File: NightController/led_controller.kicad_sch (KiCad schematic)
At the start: 22 parts, among them U301 LP5036, U302 EAST1410RGBW02, U303 EAST1410RGBW02, U304 EAST1410RGBW02, U305 EAST1410RGBW02, U306 EAST1410RGBW02, U307 EAST1410RGBW02, U308 EAST1410RGBW02, U309 EAST1410RGBW02, U310 EAST1410RGBW02

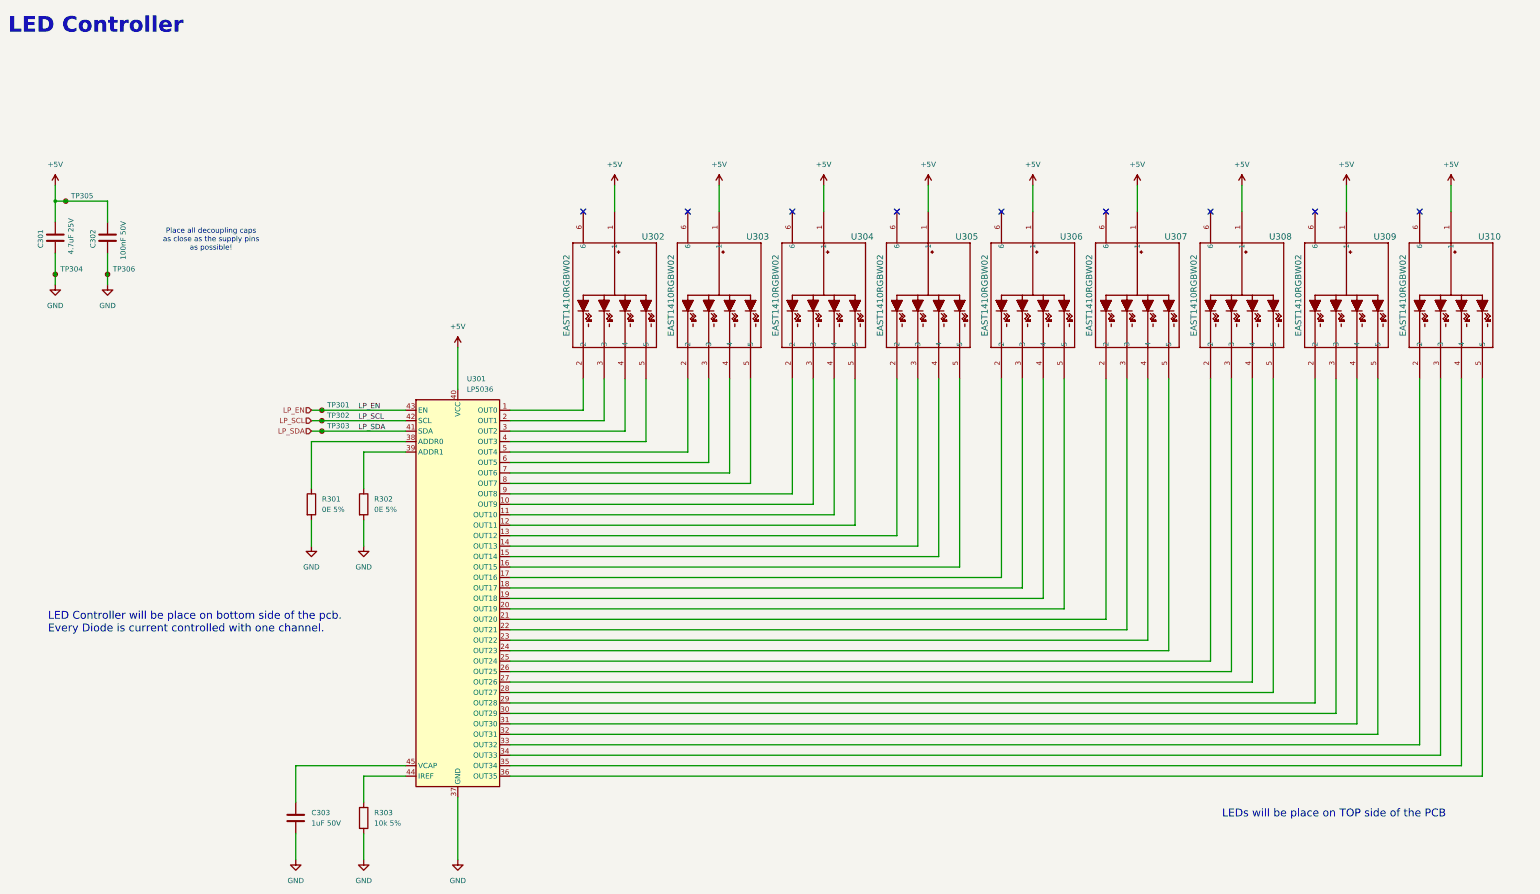
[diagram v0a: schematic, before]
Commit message: Finisched digital one
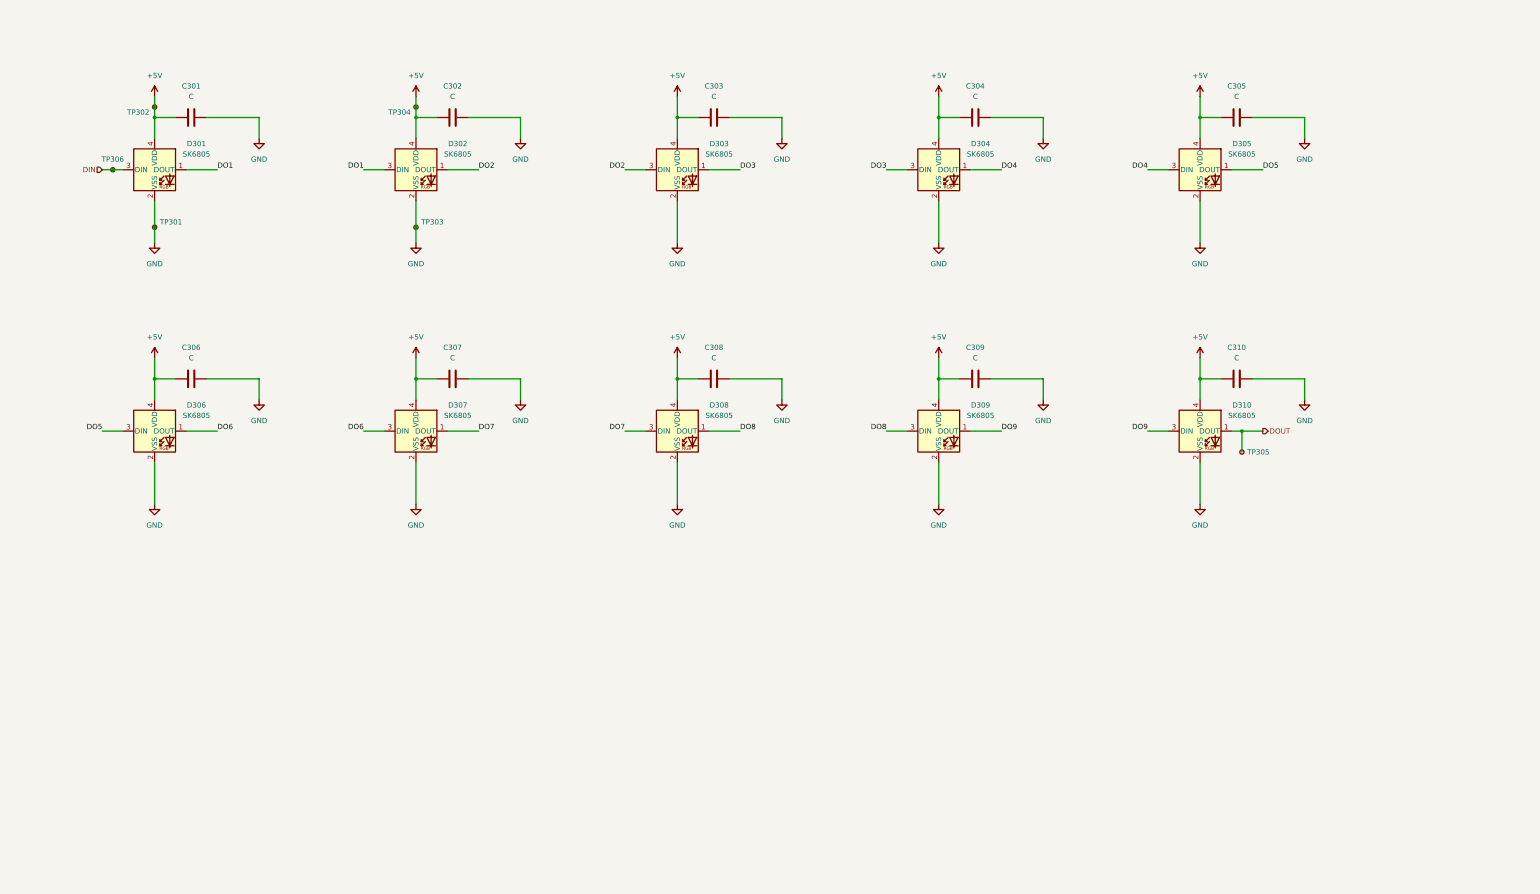
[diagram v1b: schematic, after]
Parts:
- removed R301, R302: 0E 5%, Resistor_SMD:R_0402_1005Metric_Pad0.72x0.64mm_HandSolder, symbol Device:R
- removed R303: 10k 5%, Resistor_SMD:R_0402_1005Metric_Pad0.72x0.64mm_HandSolder, symbol Device:R
- removed U301: LP5036, Package_DFN_QFN:VQFN-46-1EP_5x6mm_P0.4mm_EP2.8x3.8mm, symbol Driver_LED:LP5036
- removed U302, U303, U304, U305, U306, U307, U308, U309, U310: EAST1410RGBW02, EAST1410RGBW02:SMD_EAST1410RGBW02_EVE, symbol EAST1410RGBW02:EAST1410RGBW02
- added C304, C305, C306, C307, C308, C309, C310: C, Capacitor_SMD:C_0402_1005Metric_Pad0.74x0.62mm_HandSolder, symbol Device:C
- added D301, D302, D303, D304, D305, D306, D307, D308, D309, D310: SK6805, LED_SMD:LED_SK6805_PLCC4_2.4x2.7mm_P1.3mm, symbol LED:SK6805
- C301: value 4.7uF 25V -> C
- C302: value 100nF 50V -> C
- C303: value 1uF 50V -> C
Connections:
- net LP_EN is gone; now on net GND: TP301.1
- net LP_SCL is gone; now on net +5V: TP302.1
- net LP_SDA is gone; now on net GND: TP303.1
- net +5V: now also C303.1, TP304.1, C304.1, C305.1, C306.1, C307.1, C308.1, C309.1, C310.1, D301.4 (VDD), D302.4 (VDD), D303.4 (VDD), D304.4 (VDD), D305.4 (VDD), D306.4 (VDD), D307.4 (VDD), D308.4 (VDD), D309.4 (VDD), D310.4 (VDD); no longer TP305.1
- net GND: now also C304.2, C305.2, C306.2, C307.2, C308.2, C309.2, C310.2, D301.2 (VSS), D302.2 (VSS), D303.2 (VSS), D304.2 (VSS), D305.2 (VSS), D306.2 (VSS), D307.2 (VSS), D308.2 (VSS), D309.2 (VSS), D310.2 (VSS); no longer TP304.1, TP306.1
- new net DIN: D301.3 (DIN), TP306.1
- new net DO1: D301.1 (DOUT), D302.3 (DIN)
- new net DO2: D302.1 (DOUT), D303.3 (DIN)
- new net DO3: D303.1 (DOUT), D304.3 (DIN)
- new net DO4: D304.1 (DOUT), D305.3 (DIN)
- new net DO5: D305.1 (DOUT), D306.3 (DIN)
- new net DO6: D306.1 (DOUT), D307.3 (DIN)
- new net DO7: D307.1 (DOUT), D308.3 (DIN)
- new net DO8: D308.1 (DOUT), D309.3 (DIN)
- new net DO9: D309.1 (DOUT), D310.3 (DIN)
- new net DOUT: D310.1 (DOUT), TP305.1
- no-connect marks 9 -> 0
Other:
- note removed: "LED Controller"
- note removed: "LED Controller will be place on bottom side of the pcb. Every Diode is current controlled with one channel."
- note removed: "LEDs will be place on TOP side of the PCB"
- note removed: "Place all decoupling caps as close as the supply pins as possible!"
